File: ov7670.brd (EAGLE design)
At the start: 60.3 x 44.4 mm, 3 parts

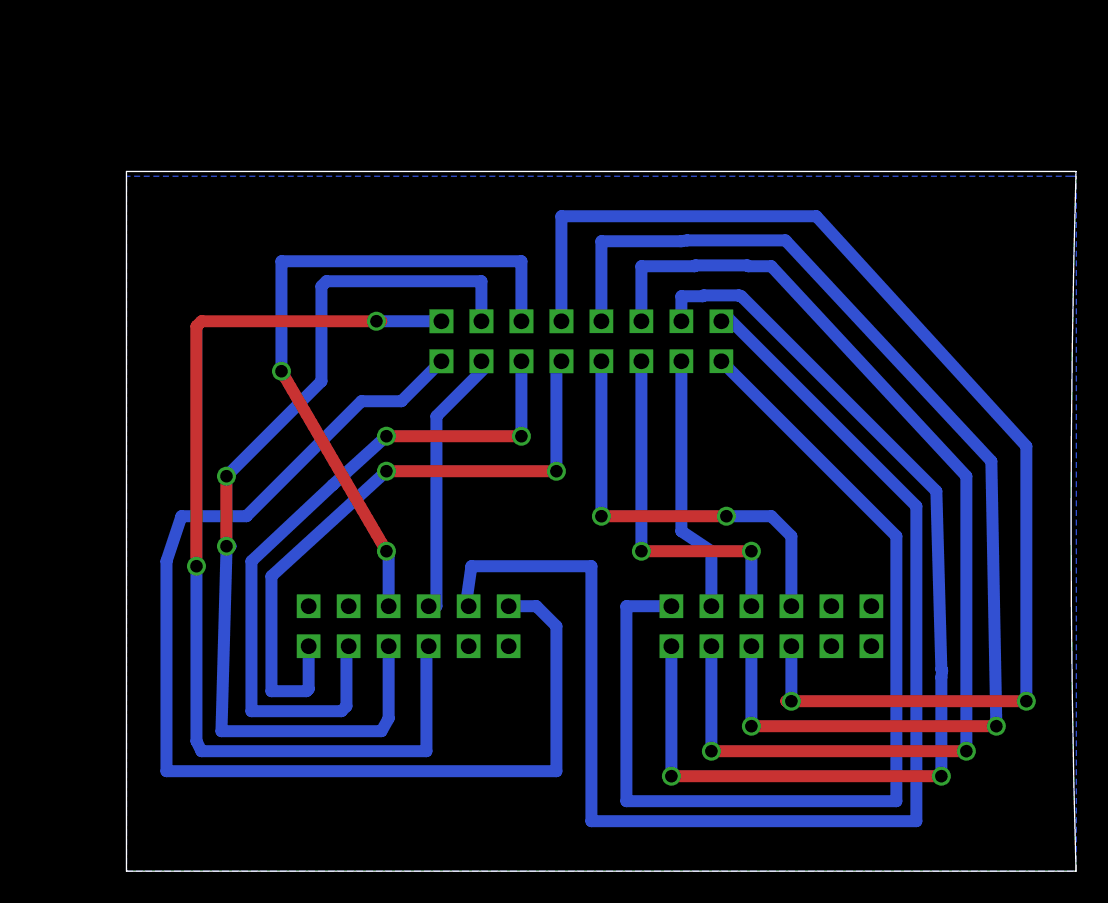
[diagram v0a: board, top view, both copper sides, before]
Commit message: temporal commit
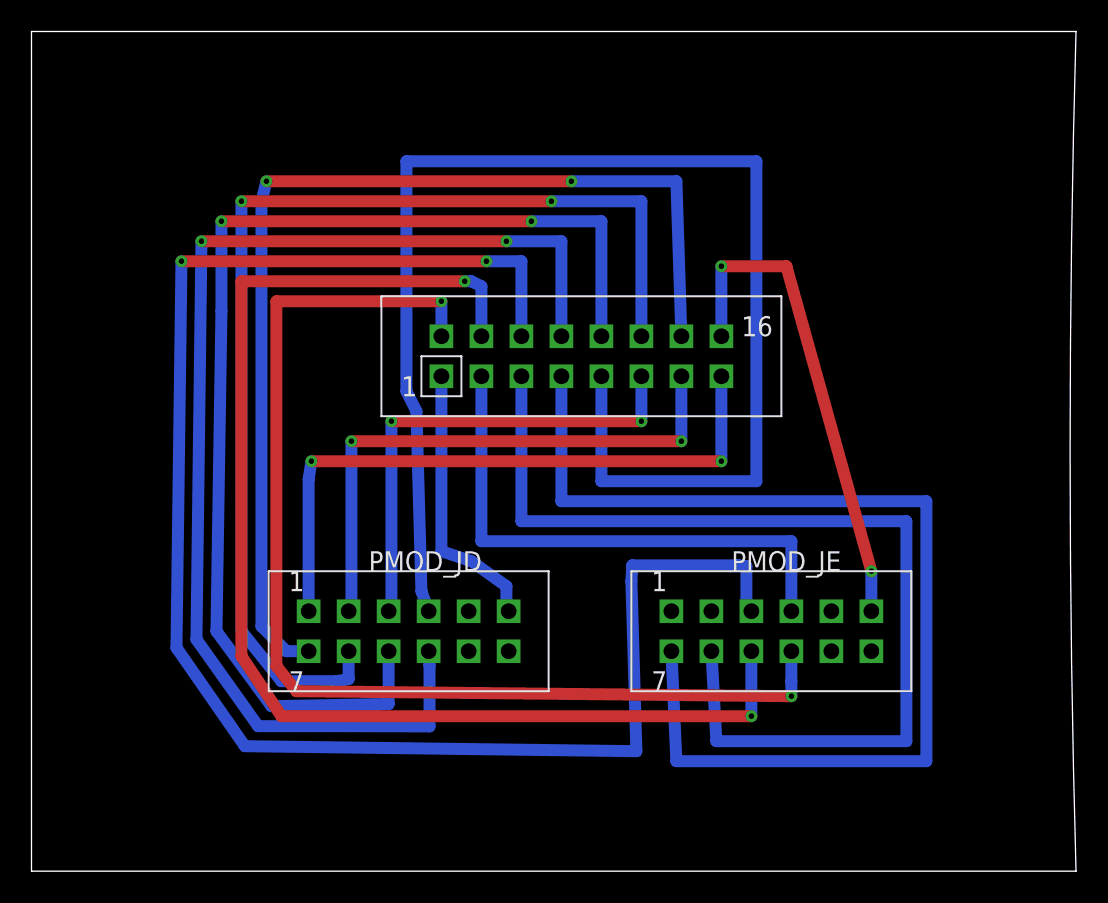
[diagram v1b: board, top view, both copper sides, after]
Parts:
- removed U$1: OV7670, ov7670:OV7670
- added D6: OV7670, ov7670:OV7670
- moved U$2 5.09 mm to (23.0, 12.7), flipped to the top, turned to 0 degrees
- moved U$3 2.86 mm to (41.0, 14.0), flipped to the top, turned to 0 degrees
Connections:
- removed net D6: U$1.D6, U$3.7
- removed net GND: U$1.GND, U$2.5
- removed net PLCK: U$1.PLCK, U$2.9
- new net N$1: D6.GND, U$3.P$6
- new net N$6: D6.D6, U$2.7
- new net PCLK: D6.PCLK, U$3.P$9
- net 3V3: now also D6.3V3; no longer U$1.3V3
- net D0: now also D6.D0, U$2.10; no longer U$1.D0, U$3.10
- net D1: now also D6.D1, U$2.4; no longer U$1.D1, U$3.4
- net D2: now also D6.D2, U$2.9; no longer U$1.D2, U$3.9
- net D3: now also D6.D3, U$2.3; no longer U$1.D3, U$3.3
- net D4: now also D6.D4, U$2.8; no longer U$1.D4, U$3.8
- net D5: now also D6.D5, U$2.2; no longer U$1.D5, U$3.2
- net D7: now also D6.D7, U$2.1; no longer U$1.D7, U$3.1
- net HREF: now also D6.HREF, U$3.P$10; no longer U$1.HREF, U$2.10
- net SCL: now also D6.SCL, U$3.P$3; no longer U$1.SCL, U$2.3
- net SDA: now also D6.SDA, U$3.P$7; no longer U$1.SDA, U$2.7
- net VSYNC: now also D6.VSYNC, U$3.P$4; no longer U$1.VSYNC, U$2.4
- net XCLK: now also D6.XCLK, U$3.P$8; no longer U$1.XCLK, U$2.8
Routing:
- net GND: track 84.6 -> 0.00 mm
- net PCLK: track 0.00 -> 80.9 mm, vias 0 -> 2
- net N$6: track 0.00 -> 67.8 mm, vias 0 -> 2
- net D6: track 66.5 -> 0.00 mm, vias 2 -> 0
- net SCL: track 42.8 -> 106.6 mm
- net D1: track 26.9 -> 87.9 mm, vias 2 -> 0
- net PLCK: track 59.7 -> 0.00 mm, vias 2 -> 0
- net 3V3: track 74.5 -> 17.5 mm
- net N$1: track 0.00 -> 31.2 mm, vias 0 -> 2
- net SDA: track 40.2 -> 70.5 mm, vias 2 -> 0
- net D7: track 64.9 -> 41.0 mm, vias 0 -> 2
- net XCLK: track 44.6 -> 65.4 mm, vias 2 -> 0
- net D5: track 16.6 -> 36.0 mm, vias 0 -> 2
- net VSYNC: track 17.5 -> 34.6 mm
- net D3: track 22.5 -> 30.9 mm
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- removed copper zone on layer 16, net GND
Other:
- board size 60.3 x 44.4 mm -> 66.3 x 53.3 mm
